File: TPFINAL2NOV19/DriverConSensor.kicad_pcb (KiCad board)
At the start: 2 copper layers, 77 x 67 mm, 53 parts, among them J1 PULS1, J2 PULS2, J3 MotorT2, J4 MotorT1, J5 VIn+12, J6 Contac12V, J7 GND, K1 Switch de Encendido, K2 FRS10CS10-12V, K3 FRS10CS10-12V, Q1 BC337, Q2 BC337, SW1 SW_DIP_x06, U1 PIC12F675-IP, U2 L78L05_TO92, U3 ACS714T-30A

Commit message: PCB
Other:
- board text added: "Grillas: 1 mm, 0,5 mm , 0,10 mm Margen: 0.3 mm Pista: 0.6 mm, 0.8mm, 1mm, 2 mm, 3mm Dist. a borde: 0.40 mm Terminacion: Estaño Plomo (Sn/Pb)"
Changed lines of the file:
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@@
   (general
     (thickness 1.6)
-    (drawings 30)
+    (drawings 31)
     (tracks 377)
     (zones 0)
@@
     (visible_elements FFFDFF7F)
     (pcbplotparams
-      (layerselection 0x31170_ffffffff)
+      (layerselection 0x11060_ffffffff)
       (usegerberextensions false)
       (usegerberattributes false)
@@
     )
   )
-  (gr_text "Las pistas que estan marcadas con máscara antisoldante \nquedan libres para ser reforzadas con estaño" (at 233.39 76.15) (layer F.CrtYd)
-    (effects (font (size 1.5 1.5) (thickness 0.3)))
+  (gr_text "Grillas: 1 mm, 0,5 mm , 0,10 mm\nMargen: 0.3 mm\nPista: 0.6 mm, 0.8mm, 1mm, 2 mm, 3mm\nDist. a borde: 0.40 mm\nTerminacion: Estaño Plomo (Sn/Pb)" (at 203.17 90.74) (layer F.CrtYd)
+    (effects (font (size 1.5 1.5) (thickness 0.3)) (justify left))
+  )
+  (gr_text "Las pistas que estan marcadas con máscara antisoldante \nquedan libres para ser reforzadas con estaño" (at 203.61 75.79) (layer F.CrtYd)
+    (effects (font (size 1.5 1.5) (thickness 0.3)) (justify left))
   )
   (gr_line (start 139.2 77.575) (end 135.8 77.625) (layer B.Mask) (width 3))
@@
     (effects (font (size 1.8 1.8) (thickness 0.25)))
   )
-  (gr_text "El pad GND1 y GND2 es para colocar un cable en dichos \nlugares para reforzar la union de ambas masas, que se \nrealiza en el relleno de cobre por un lugar estrecho" (at 200.25 63.775) (layer F.CrtYd)
+  (gr_text "El pad GND1 y GND2 es para colocar un cable en dichos \nlugares para reforzar la union de ambas masas, que se \nrealiza en el relleno de cobre por un lugar estrecho" (at 203.17 64.35) (layer F.CrtYd)
     (effects (font (size 1.5 1.5) (thickness 0.3)) (justify left))
   )

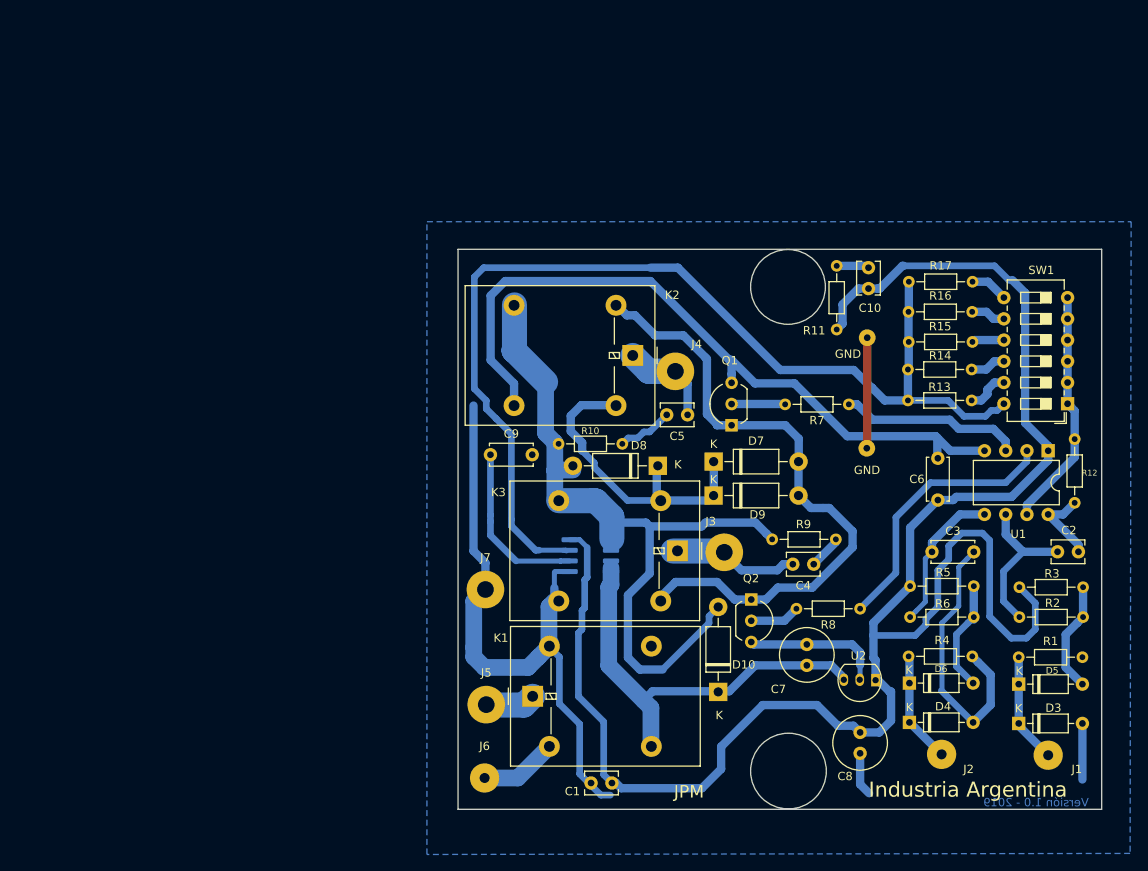
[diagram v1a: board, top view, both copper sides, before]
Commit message: PCB_Final
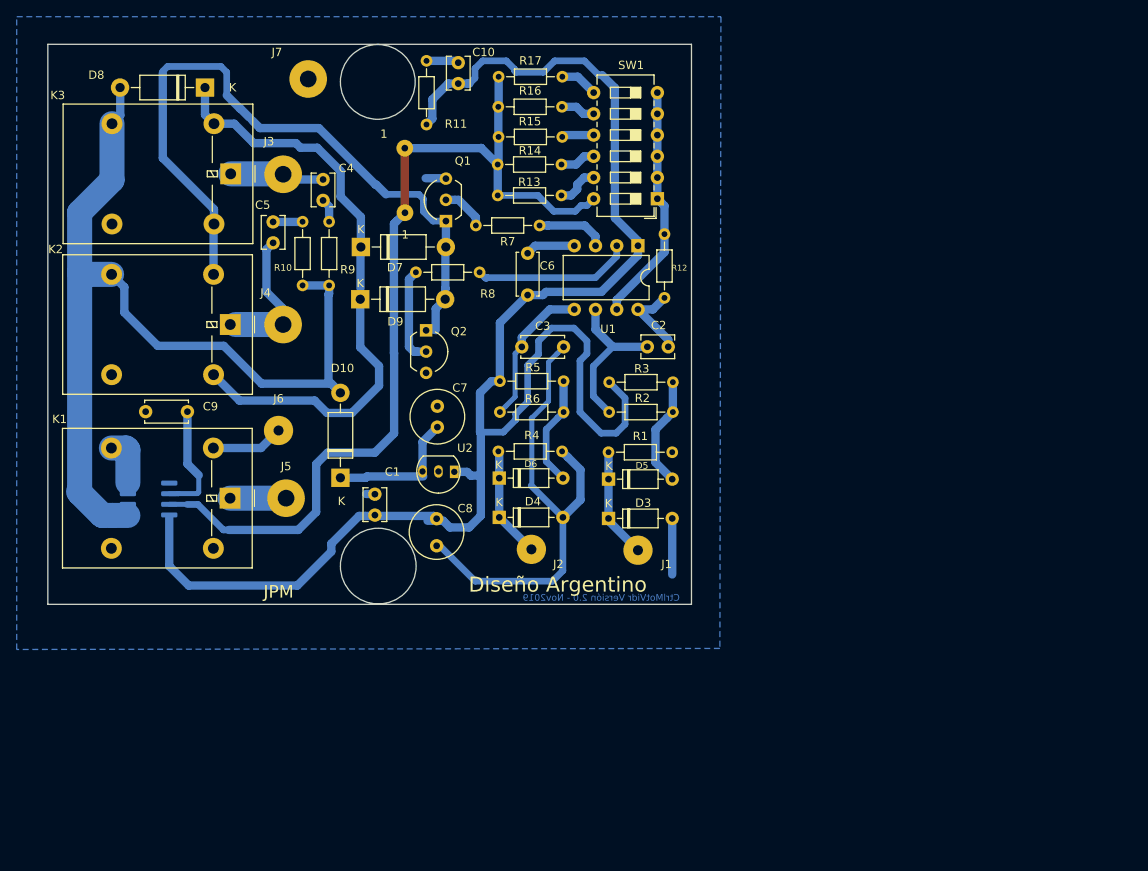
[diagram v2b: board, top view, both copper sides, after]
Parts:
- moved C4 73.1 mm to (96.8, 57.1), turned to 90 degrees
- moved R9 71.5 mm to (97.6, 59.7), turned to 270 degrees
- moved D8 70.6 mm to (82.7, 43.6)
- moved K3 69.9 mm to (85.8, 54.0)
- moved J3 69.5 mm to (92.1, 54.0)
- moved J7 64.6 mm to (95.1, 42.6)
- moved 1 62.0 mm to (106.7, 58.6)
- moved R8 60.8 mm to (115.6, 65.8)
- moved 1 59.8 mm to (106.6, 50.9)
- moved C8 56.6 mm to (110.4, 95.6)
- moved U2 56.2 mm to (111.9, 89.6)
- moved R2 54.9 mm to (138.7, 82.5)
- moved R11 54.9 mm to (109.2, 48.1)
- moved R12 54.9 mm to (137.7, 61.2)
- moved R3 54.9 mm to (138.7, 78.9)
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- renumbered GND to 1
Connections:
- 1 pad 2: GND -> Net-(R13-Pad1)
- 1 pad 1: GND -> Net-(R13-Pad1)
- C7 pad 1: +12V -> Net-(C7-Pad1)
- D10 pad 1: +12V -> Net-(C7-Pad1)
- J5 pad 1: Net-(J5-Pad1) -> +12V
- K1 pad 1: Net-(J5-Pad1) -> +12V
- K1 pad 3: +12V -> Net-(K1-Pad3)
- U2 pad 3: +12V -> Net-(C7-Pad1)
- U3 pad 3: +12V -> Net-(K1-Pad3)
- U3 pad 4: +12V -> Net-(K1-Pad3)
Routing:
- net GND: track 253.1 -> 86.6 mm
- net +12V: track 50.2 -> 6.70 mm
- net Net-(D7-Pad1): track 37.0 -> 71.0 mm
- net /Relay2y3_NA: track 90.0 -> 117.1 mm
- net +5V: track 214.7 -> 193.6 mm
- net Net-(C7-Pad1): track 0.00 -> 16.0 mm
- net Net-(R13-Pad1): track 125.5 -> 110.1 mm
- net /GP5(PIN3PIC): track 32.4 -> 19.1 mm
- net /GP4(PIN2PIC): track 21.7 -> 8.36 mm
- net Net-(D7-Pad2): track 77.2 -> 85.2 mm
- net Net-(C9-Pad1): track 20.4 -> 13.8 mm
- net Net-(J5-Pad1): track 6.38 -> 0.00 mm
- net Net-(K1-Pad3): track 0.00 -> 5.99 mm
- net Net-(Q2-Pad2): track 6.00 -> 11.5 mm
- net Net-(C4-Pad2): track 17.2 -> 12.6 mm
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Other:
- rule via_min_size: 0.4 -> 0.3
- board text added: "AGUJERO DE SUJECIÓN : Esta placa iria en una caja de plastico que posee dos cilindros pasantes para sostener la misma, que son los dos agujeros representados por circulos. Si queda u zoa fragil como mecionó en la corrección pero es por que el case donde va ir alojada ya esta hecho, se busca reemplazar una placa ya hecha actualmente con las mismas medidas de forma"
- board text added: "CtrlMotVidr Versión 2.0 - Nov2019"
- board text added: "Diseño Argentino"
- board text added: "Grillas: 1 mm, 0,5 mm , 0,10 mm Margen: 0.3 mm Pista: 0.6 mm, 0.8mm, 1mm, 2 mm, 3mm Dist. a borde: 0.40 mm Terminacion: HASL Fabricante: Mayer"
- board text added: "Q1 y Q2; si bien en el esquematico se menciona aclaro aca su función, los mismos estan en paralelo en cuanto a colector-emisor, pero la base de cada uno esta conectada a la salida de los GPIO para que puedan ser activas o desactivados segun una logica que es la siguientes: Cuando se activa un GPIO mueve un relay por donde queda a 12v y de ahi va a lo borne del motor, el otro motor esta al otro re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"
- board text added: "SMD :la razon de uso de un componente SMD es que este modelo en particular es un sensor de corriente de 30A para uso en el rubro automotor solo con encapsulado smd se consigue. No se opto por hacer smd en su totalidad por falta de experiencia, pero se realizará a futuro para una mejora de la presente versión"
- board text removed: "Grillas: 1 mm, 0,5 mm , 0,10 mm Margen: 0.3 mm Pista: 0.6 mm, 0.8mm, 1mm, 2 mm, 3mm Dist. a borde: 0.40 mm Terminacion: Estaño Plomo (Sn/Pb)"
- board text removed: "Industria Argentina"
- board text removed: "Versión 1.0 - 2019"
